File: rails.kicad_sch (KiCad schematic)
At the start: 93 parts, among them Q15 2N7002, U13 LM61460AASQRJRRQ1, U14 LM61460AASQRJRRQ1, U15 TPS259474ARPWR, U16 SN74LVC1G74, Y2 SX1M4.000M10F30TNN

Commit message: assign lcsc part numbers
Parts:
- R113, R119, R132: LCSC Part C2902636 -> C54951138
- R114, R120: LCSC Part C1883546 -> C54530672
- R128: LCSC Part (none) -> C100525
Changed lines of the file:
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@@
 			)
 		)
-		(property "LCSC Part" ""
+		(property "LCSC Part" "C100525"
 			(at 219.71 87.63 0)
 			(hide yes)
@@
 			)
 		)
-		(property "LCSC Part" "C2902636"
+		(property "LCSC Part" "C54951138"
 			(at 132.08 60.96 0)
 			(hide yes)
@@
 			)
 		)
-		(property "LCSC Part" "C2902636"
+		(property "LCSC Part" "C54951138"
 			(at 256.54 132.08 0)
 			(hide yes)
@@
 			)
 		)
-		(property "LCSC Part" "C2902636"
+		(property "LCSC Part" "C54951138"
 			(at 120.65 144.78 0)
 			(hide yes)
@@
 			)
 		)
-		(property "LCSC Part" "C1883546"
+		(property "LCSC Part" "C54530672"
 			(at 127 158.75 0)
 			(hide yes)
@@
 			)
 		)
-		(property "LCSC Part" "C1883546"
+		(property "LCSC Part" "C54530672"
 			(at 142.24 74.93 0)
 			(hide yes)

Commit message: new part numbers for out of stock components
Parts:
- R129: LCSC Part C861797 -> C705755
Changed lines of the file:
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@@
 			)
 		)
-		(property "LCSC Part" "C861797"
+		(property "LCSC Part" "C705755"
 			(at 231.14 66.04 0)
 			(hide yes)
@@
 			(at 231.14 66.04 0)
 			(hide yes)
+			(show_name no)
+			(do_not_autoplace no)
+			(effects
+				(font
+					(size 1.27 1.27)
+				)
+			)
+		)
+		(property "Capacitor Rating" ""
+			(at 231.14 66.04 0)
+			(hide yes)

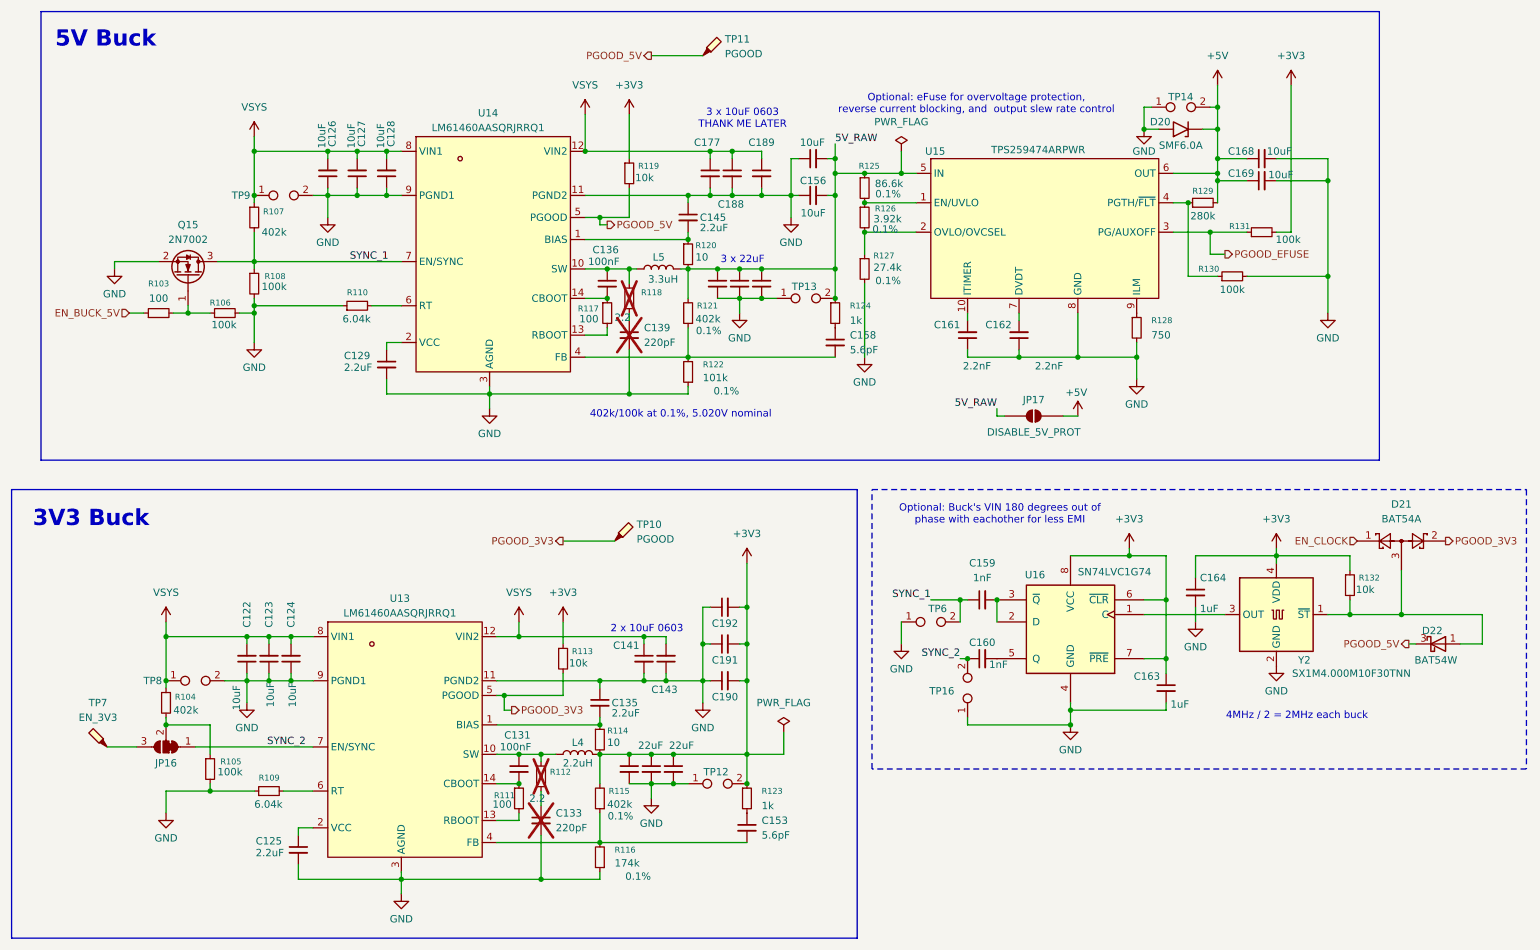
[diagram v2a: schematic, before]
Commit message: backup before switching to kicad-nightly
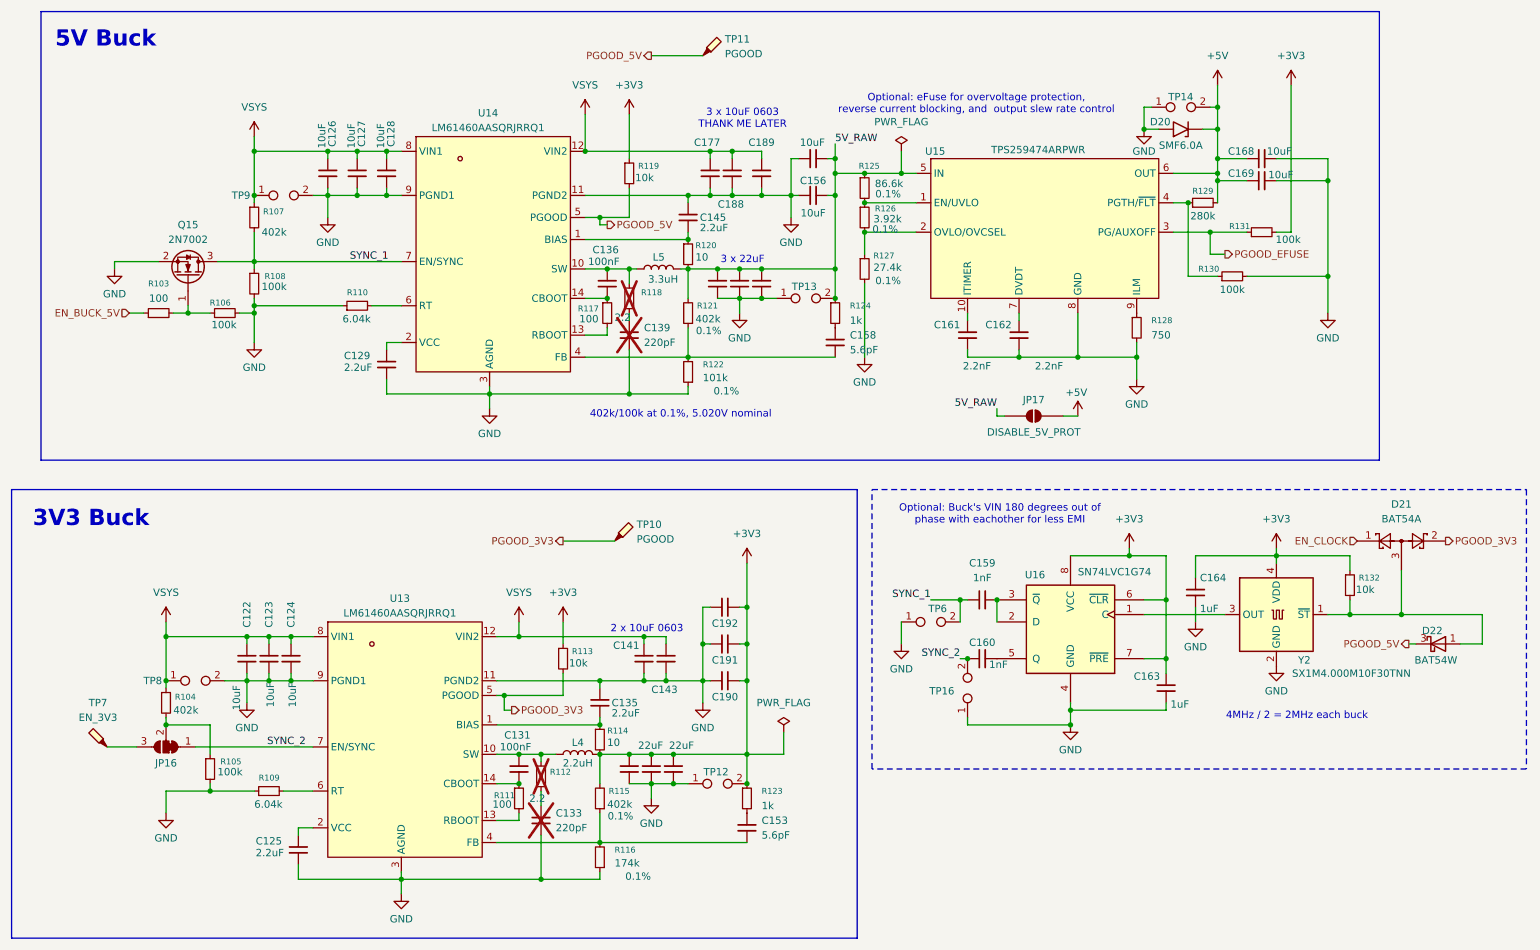
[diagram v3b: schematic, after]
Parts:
- TP7: now left out of the parts list
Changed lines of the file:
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@@
 		(body_style 1)
 		(exclude_from_sim no)
-		(in_bom yes)
+		(in_bom no)
 		(on_board yes)
 		(in_pos_files yes)
